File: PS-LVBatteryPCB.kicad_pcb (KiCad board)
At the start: 2 copper layers, 30.8 x 38.8 mm, 11 parts, among them J1 NTC_01, J2 NTC_02, J3 NTC_OUT, J4 SUPP+, J5 SUPP_GND, J6 SUPP_FUSE

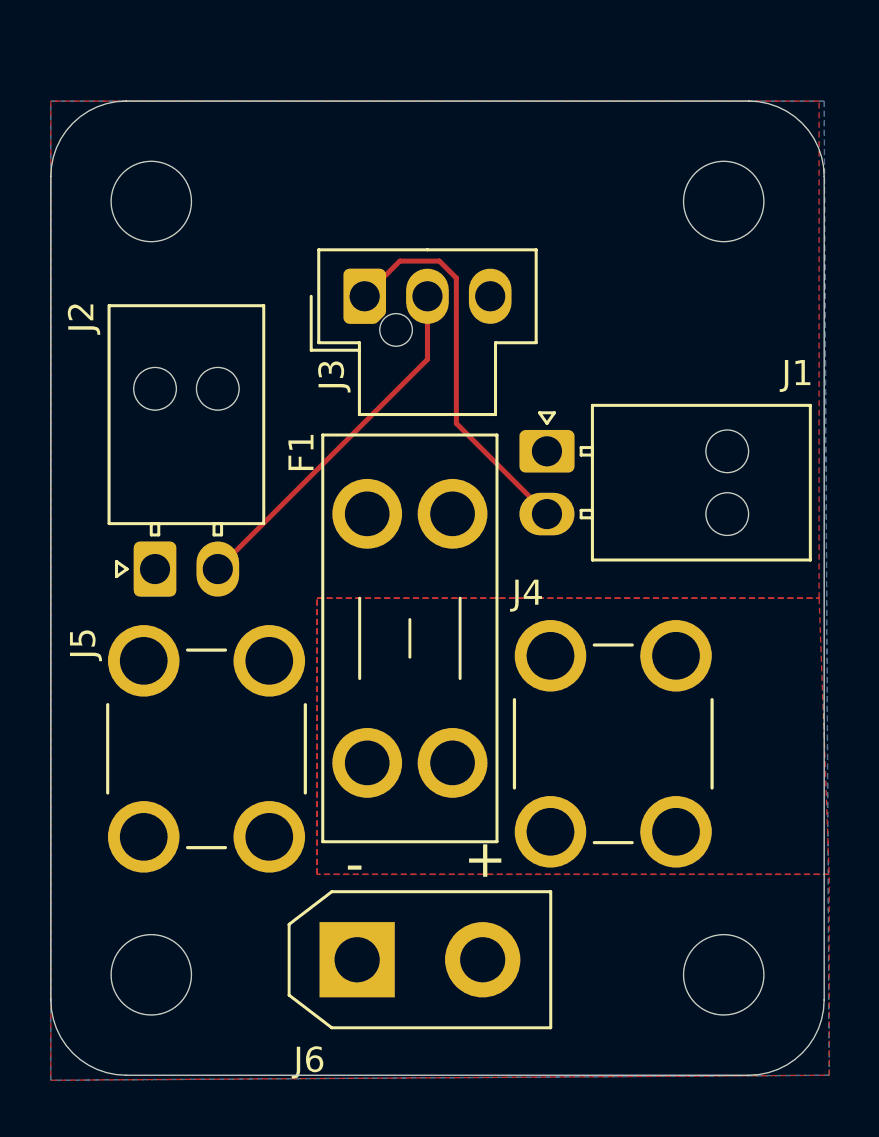
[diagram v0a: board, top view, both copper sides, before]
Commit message: reorganize and added SOME 3D models
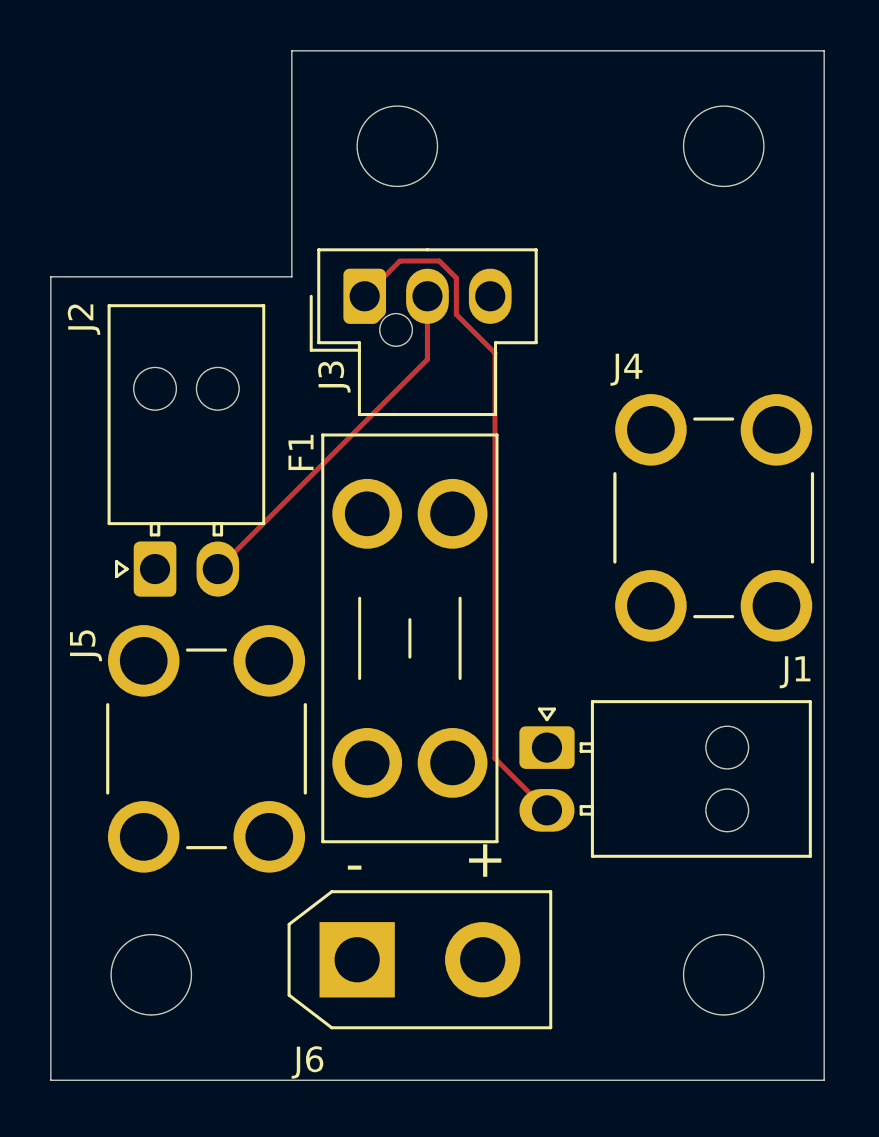
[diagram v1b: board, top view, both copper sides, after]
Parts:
- moved J1 11.8 mm to (145.0, 104.2)
- moved REF** 10.0 mm to (139.0, 80.2)
- moved J4 9.85 mm to (151.6, 95.0)
- moved REF** 2.20 mm to (152.0, 80.2)
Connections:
- F1 pad 1: /SUPP_FUSE+ -> /SUPP+
- F1 pad 2: /SUPP+ -> /SUPP_FUSE+
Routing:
- net Net-(J1-Pin_2): track 15.4 -> 27.2 mm
- removed copper zone on F.Cu, net /SUPP+
- removed copper zone on F.Cu, net /SUPP_FUSE+
- removed copper zone on B.Cu, net /SUPP_GND
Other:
- board size 30.8 x 38.8 mm -> 30.8 x 41 mm
